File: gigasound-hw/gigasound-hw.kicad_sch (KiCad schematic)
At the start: 14 parts, among them J1 Conn_01x04_Socket, J2 Conn_01x05_Socket, SW1 PLAY, SW2 STOP, SW3 MODE, U1 STM32F401RETx, Y1 8MHz

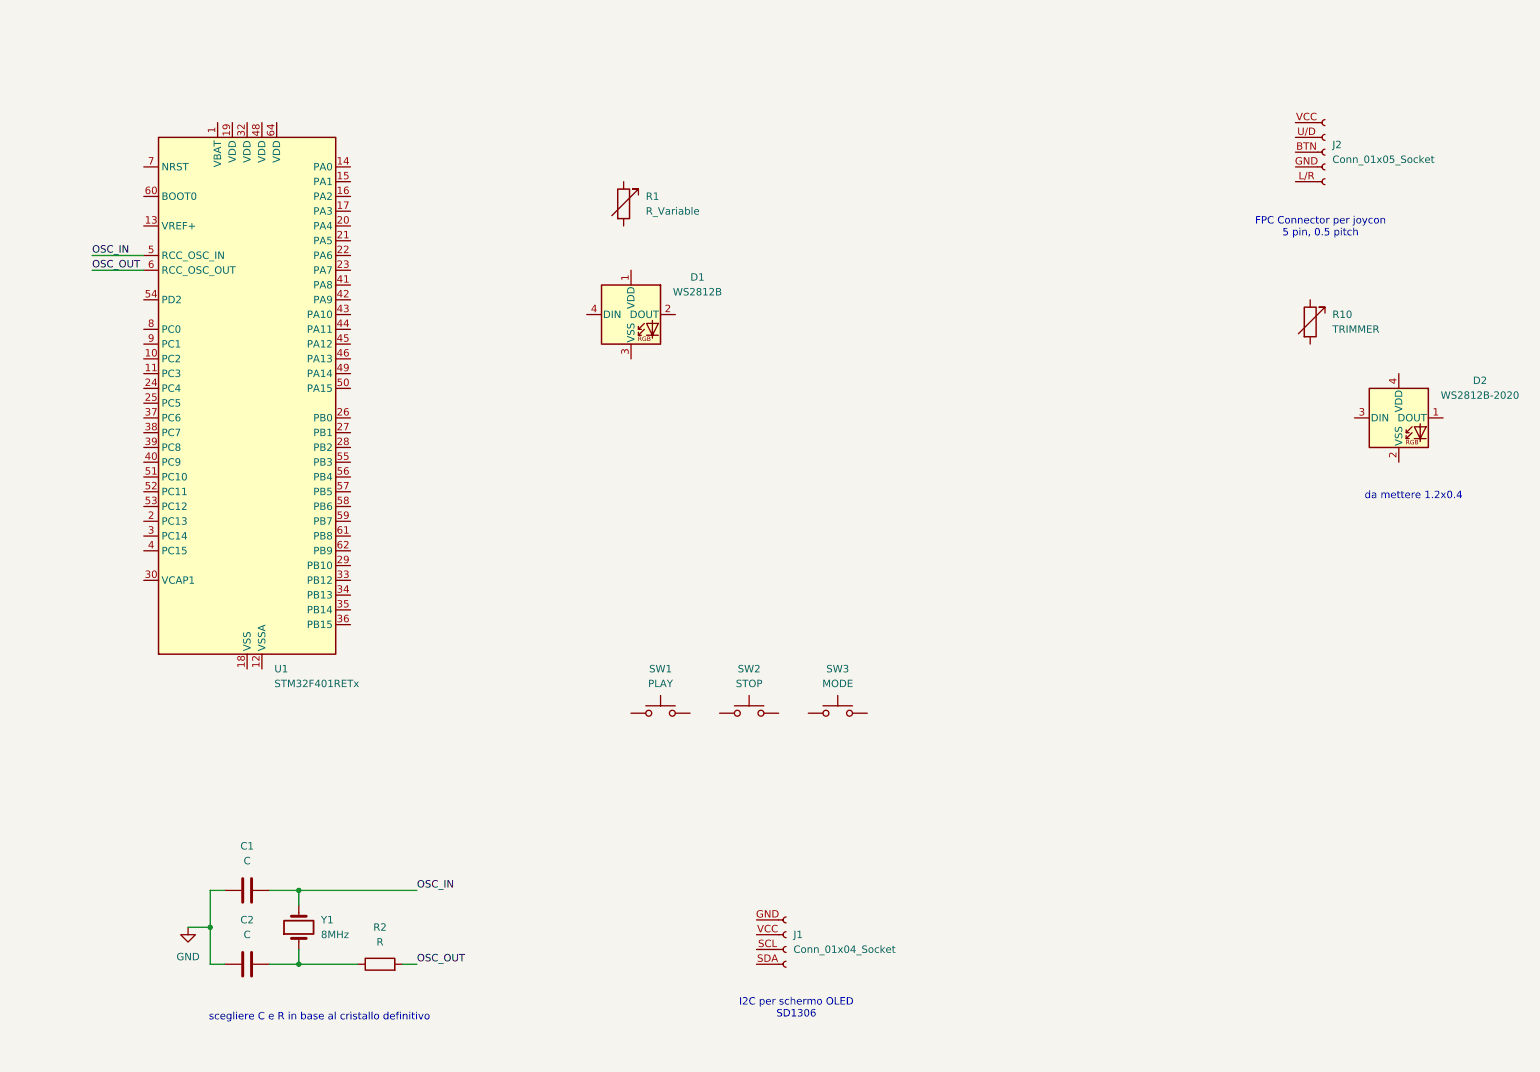
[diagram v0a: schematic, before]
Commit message: progress hw schematic
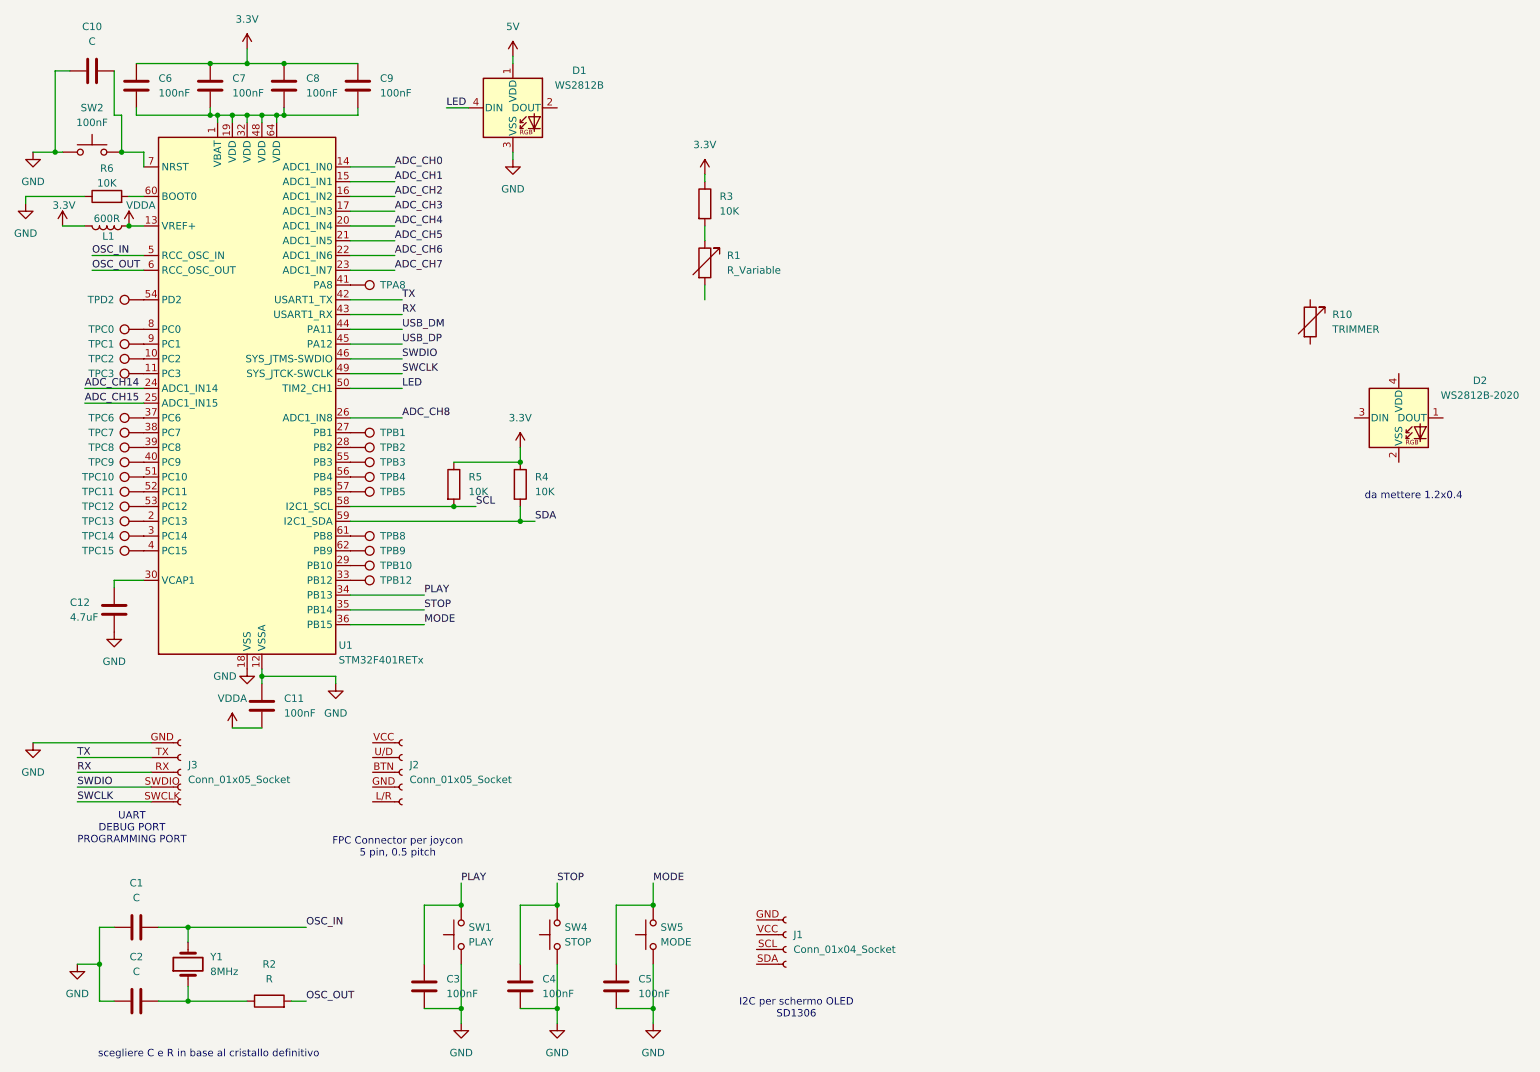
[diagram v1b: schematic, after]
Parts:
- removed SW3: MODE, symbol Switch:SW_Push
- added C10: C, symbol Device:C
- added C11, C3, C4, C5, C6, C7, C8, C9: 100nF, symbol Device:C
- added C12: 4.7uF, symbol Device:C
- added J3: Conn_01x05_Socket, symbol Connector:Conn_01x05_Socket
- added L1: 600R, symbol Device:L
- added R3, R4, R5, R6: 10K, symbol Device:R
- added SW4: STOP, symbol Switch:SW_Push
- added SW5: MODE, symbol Switch:SW_Push
- added TPA8, TPB1, TPB10, TPB12, TPB2, TPB3, TPB4, TPB5, TPB8, TPB9, TPC0, TPC1, TPC10, TPC11, TPC12, TPC13, TPC14, TPC15, TPC2, TPC3, TPC6, TPC7, TPC8, TPC9, TPD2: ~, TestPoint:TestPoint_Pad_D1.0mm, symbol Connector:TestPoint
- SW2: value STOP -> 100nF
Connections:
- net GND: now also D1.3 (VSS), SW1.1, SW2.1, U1.12 (VSSA), U1.18 (VSS), U1.31 (VSS), U1.47 (VSS), U1.63 (VSS), C10.1, C11.1, C12.1, C3.2, C4.2, C5.2, J3.GND, R6.1, SW4.1, SW5.1
- net 5V: now reaches D1.1 (VDD)
- net LED: now reaches D1.4 (DIN)
- net LED: now also U1.50 (PA15)
- net PLAY: now reaches SW1.2
- net PLAY: now also U1.34 (PB13), C3.1
- net at SW2.2: now also U1.7 (NRST), C10.2
- net at R1.1: now also R3.2
- net at U1.1 (VBAT): now also U1.19 (VDD), U1.32 (VDD), U1.48 (VDD), U1.64 (VDD), C6.2, C7.2, C8.2, C9.2
- net at U1.10 (PC2): now also TPC2.1
- net at U1.11 (PC3): now also TPC3.1
- net VDDA: now reaches U1.13 (VREF+)
- net VDDA: now also C11.2, L1.1
- net ADC_CH0: now reaches U1.14 (PA0)
- net ADC_CH1: now reaches U1.15 (PA1)
- net ADC_CH2: now reaches U1.16 (PA2)
- net ADC_CH3: now reaches U1.17 (PA3)
- net at U1.2 (PC13): now also TPC13.1
- net ADC_CH4: now reaches U1.20 (PA4)
- net ADC_CH5: now reaches U1.21 (PA5)
- net ADC_CH6: now reaches U1.22 (PA6)
- net ADC_CH7: now reaches U1.23 (PA7)
- net ADC_CH14: now reaches U1.24 (PC4)
- net ADC_CH15: now reaches U1.25 (PC5)
- net ADC_CH8: now reaches U1.26 (PB0)
- net at U1.27 (PB1): now also TPB1.1
- net at U1.28 (PB2): now also TPB2.1
- net at U1.29 (PB10): now also TPB10.1
- net at U1.3 (PC14): now also TPC14.1
- net at U1.30 (VCAP1): now also C12.2
- net at U1.33 (PB12): now also TPB12.1
- net STOP: now reaches U1.35 (PB14)
- net STOP: now also C4.1, SW4.2
- net MODE: now reaches U1.36 (PB15)
- net MODE: now also C5.1, SW5.2
- net at U1.37 (PC6): now also TPC6.1
- net at U1.38 (PC7): now also TPC7.1
- net at U1.39 (PC8): now also TPC8.1
- net at U1.4 (PC15): now also TPC15.1
- net at U1.40 (PC9): now also TPC9.1
- net at U1.41 (PA8): now also TPA8.1
- net TX: now reaches U1.42 (PA9)
- net TX: now also J3.TX
- net RX: now reaches U1.43 (PA10)
- net RX: now also J3.RX
- net USB_DM: now reaches U1.44 (PA11)
- net USB_DP: now reaches U1.45 (PA12)
- net SWDIO: now reaches U1.46 (PA13)
- net SWDIO: now also J3.SWDIO
- net SWCLK: now reaches U1.49 (PA14)
- net SWCLK: now also J3.SWCLK
- net at U1.51 (PC10): now also TPC10.1
- net at U1.52 (PC11): now also TPC11.1
- net at U1.53 (PC12): now also TPC12.1
- net at U1.54 (PD2): now also TPD2.1
- net at U1.55 (PB3): now also TPB3.1
- net at U1.56 (PB4): now also TPB4.1
- net at U1.57 (PB5): now also TPB5.1
- net SCL: now reaches U1.58 (PB6)
- net SCL: now also R5.2
- net SDA: now reaches U1.59 (PB7)
- net SDA: now also R4.2
- net at U1.60 (BOOT0): now also R6.2
- net at U1.61 (PB8): now also TPB8.1
- net at U1.62 (PB9): now also TPB9.1
- net at U1.8 (PC0): now also TPC0.1
- net at U1.9 (PC1): now also TPC1.1
- new net 3.3V: C6.1, C7.1, C8.1, C9.1, L1.2, R3.1, R4.1, R5.1
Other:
- note added: "UART DEBUG PORT PROGRAMMING PORT"
- company: (none) -> Poliba
- title: (none) -> GigaSound-MIDI
- moved on the sheet: C1, C2, D1, J2, R1, R2, SW1, Y1
